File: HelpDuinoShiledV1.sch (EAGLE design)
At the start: 30 parts

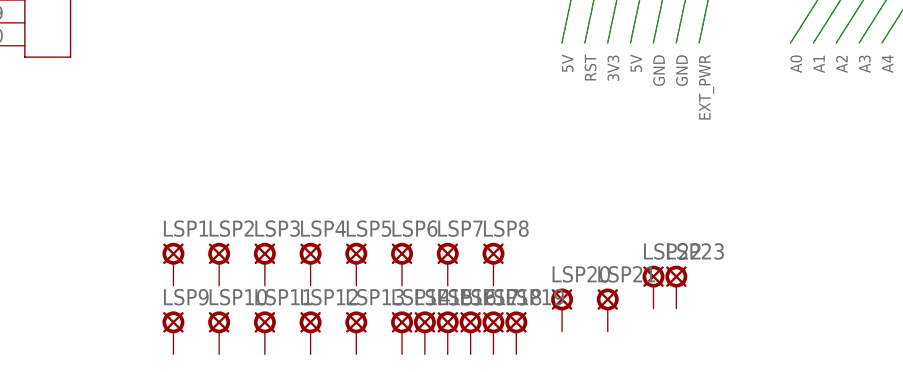
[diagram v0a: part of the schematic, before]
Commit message: adding traces
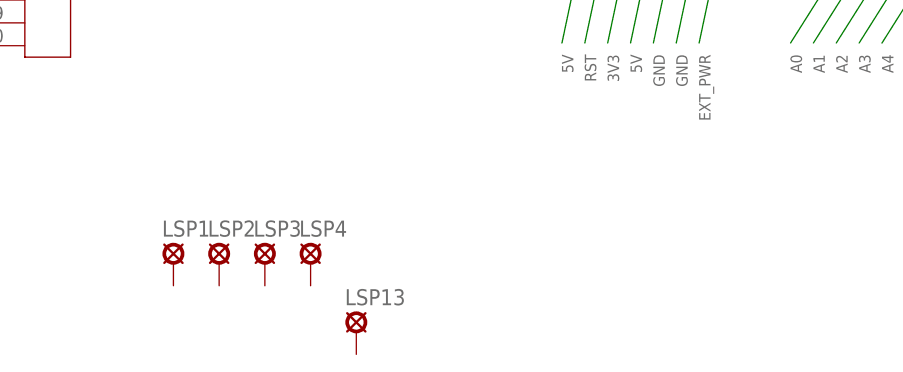
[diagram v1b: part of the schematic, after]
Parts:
- removed LSP10, LSP11, LSP12, LSP14, LSP15, LSP16, LSP17, LSP18, LSP19, LSP20, LSP21, LSP22, LSP23, LSP5, LSP6, LSP7, LSP8, LSP9: SE13, solpad:SE13
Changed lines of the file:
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@@
 <part name="LSP3" library="solpad" deviceset="SE13" device=""/>
 <part name="LSP4" library="solpad" deviceset="SE13" device=""/>
-<part name="LSP5" library="solpad" deviceset="SE13" device=""/>
-<part name="LSP6" library="solpad" deviceset="SE13" device=""/>
-<part name="LSP7" library="solpad" deviceset="SE13" device=""/>
-<part name="LSP8" library="solpad" deviceset="SE13" device=""/>
-<part name="LSP9" library="solpad" deviceset="SE13" device=""/>
-<part name="LSP10" library="solpad" deviceset="SE13" device=""/>
-<part name="LSP11" library="solpad" deviceset="SE13" device=""/>
-<part name="LSP12" library="solpad" deviceset="SE13" device=""/>
 <part name="LSP13" library="solpad" deviceset="SE13" device=""/>
-<part name="LSP14" library="solpad" deviceset="SE13" device=""/>
-<part name="LSP15" library="solpad" deviceset="SE13" device=""/>
-<part name="LSP16" library="solpad" deviceset="SE13" device=""/>
-<part name="LSP17" library="solpad" deviceset="SE13" device=""/>
-<part name="LSP18" library="solpad" deviceset="SE13" device=""/>
-<part name="LSP19" library="solpad" deviceset="SE13" device=""/>
-<part name="LSP20" library="solpad" deviceset="SE13" device=""/>
-<part name="LSP21" library="solpad" deviceset="SE13" device=""/>
-<part name="LSP22" library="solpad" deviceset="SE13" device=""/>
-<part name="LSP23" library="solpad" deviceset="SE13" device=""/>
 </parts>
 <sheets>
@@
 <instance part="LSP3" gate="1" x="58.42" y="-25.4"/>
 <instance part="LSP4" gate="1" x="63.5" y="-25.4"/>
-<instance part="LSP5" gate="1" x="68.58" y="-25.4"/>
-<instance part="LSP6" gate="1" x="73.66" y="-25.4"/>
-<instance part="LSP7" gate="1" x="78.74" y="-25.4"/>
-<instance part="LSP8" gate="1" x="83.82" y="-25.4"/>
-<instance part="LSP9" gate="1" x="48.26" y="-33.02"/>
-<instance part="LSP10" gate="1" x="53.34" y="-33.02"/>
-<instance part="LSP11" gate="1" x="58.42" y="-33.02"/>
-<instance part="LSP12" gate="1" x="63.5" y="-33.02"/>
 <instance part="LSP13" gate="1" x="68.58" y="-33.02"/>
-<instance part="LSP14" gate="1" x="73.66" y="-33.02"/>
-<instance part="LSP15" gate="1" x="76.2" y="-33.02"/>
-<instance part="LSP16" gate="1" x="78.74" y="-33.02"/>
-<instance part="LSP17" gate="1" x="81.28" y="-33.02"/>
-<instance part="LSP18" gate="1" x="83.82" y="-33.02"/>
-<instance part="LSP19" gate="1" x="86.36" y="-33.02"/>
-<instance part="LSP20" gate="1" x="91.44" y="-30.48"/>
-<instance part="LSP21" gate="1" x="96.52" y="-30.48"/>
-<instance part="LSP22" gate="1" x="101.6" y="-27.94"/>
-<instance part="LSP23" gate="1" x="104.14" y="-27.94"/>
 </instances>
 <busses>
